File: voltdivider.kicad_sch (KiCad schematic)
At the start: 20 parts, among them J1 Conn_01x01_Pin, J7 Conn_01x01_Pin, J8 Conn_01x01_Pin, SW1 SW_Rotary_1x8_MP

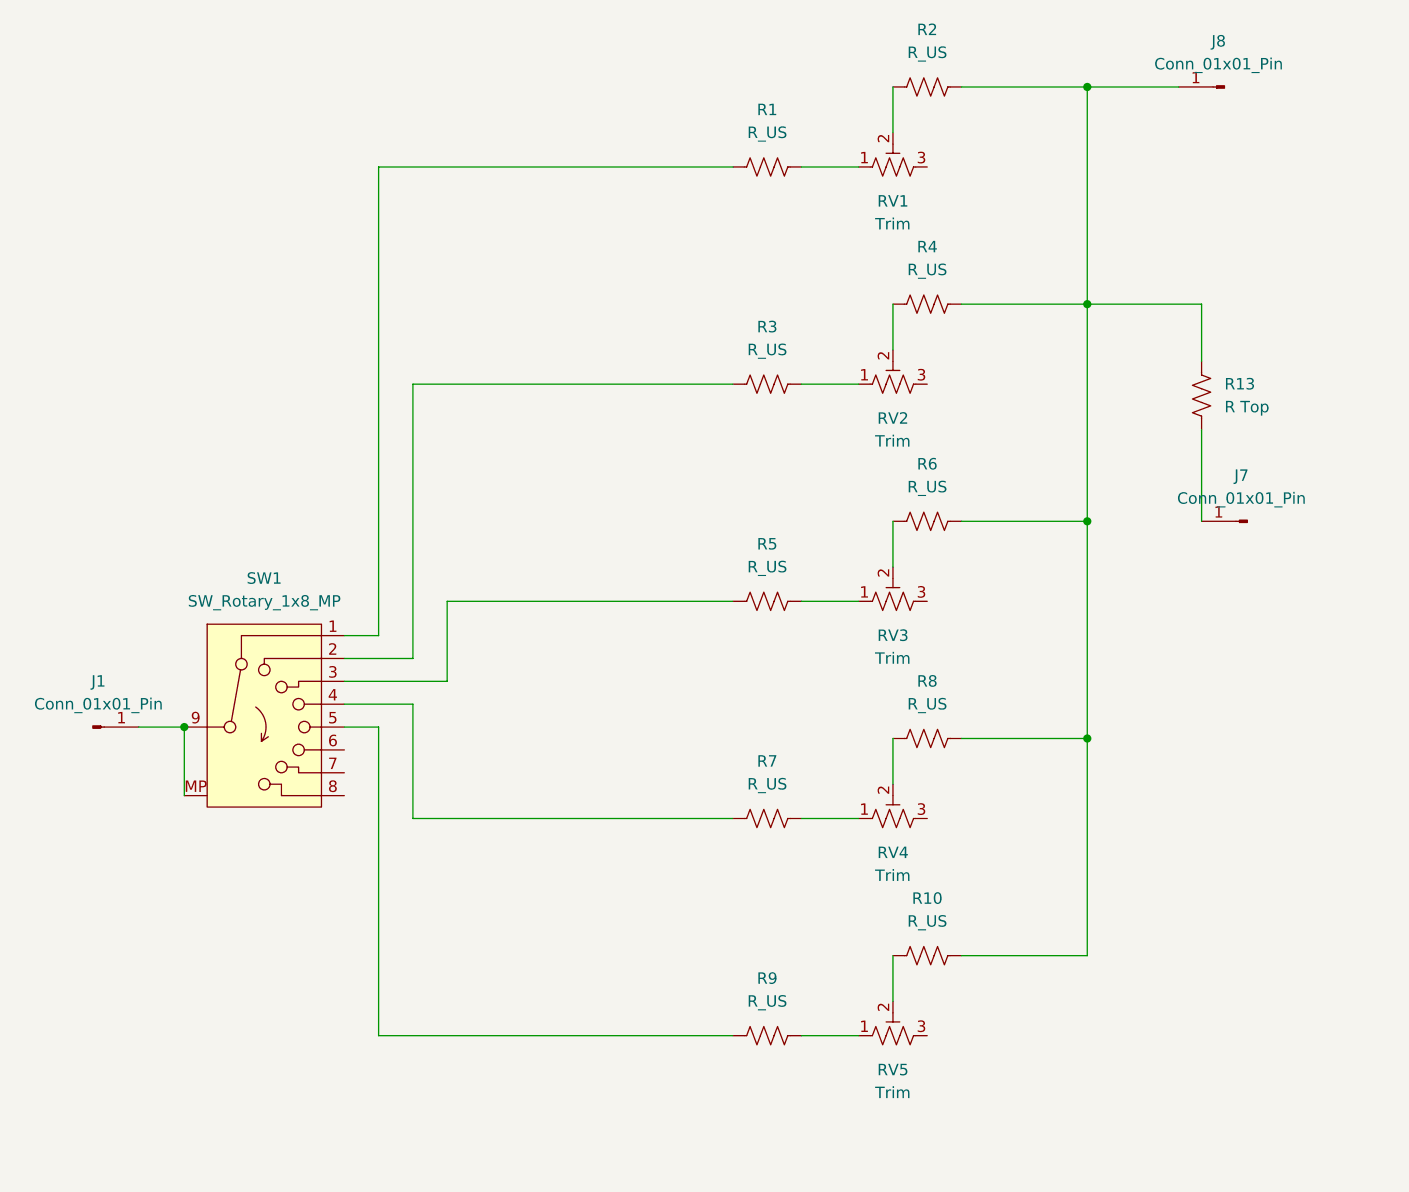
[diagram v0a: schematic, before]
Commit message: creating documentation
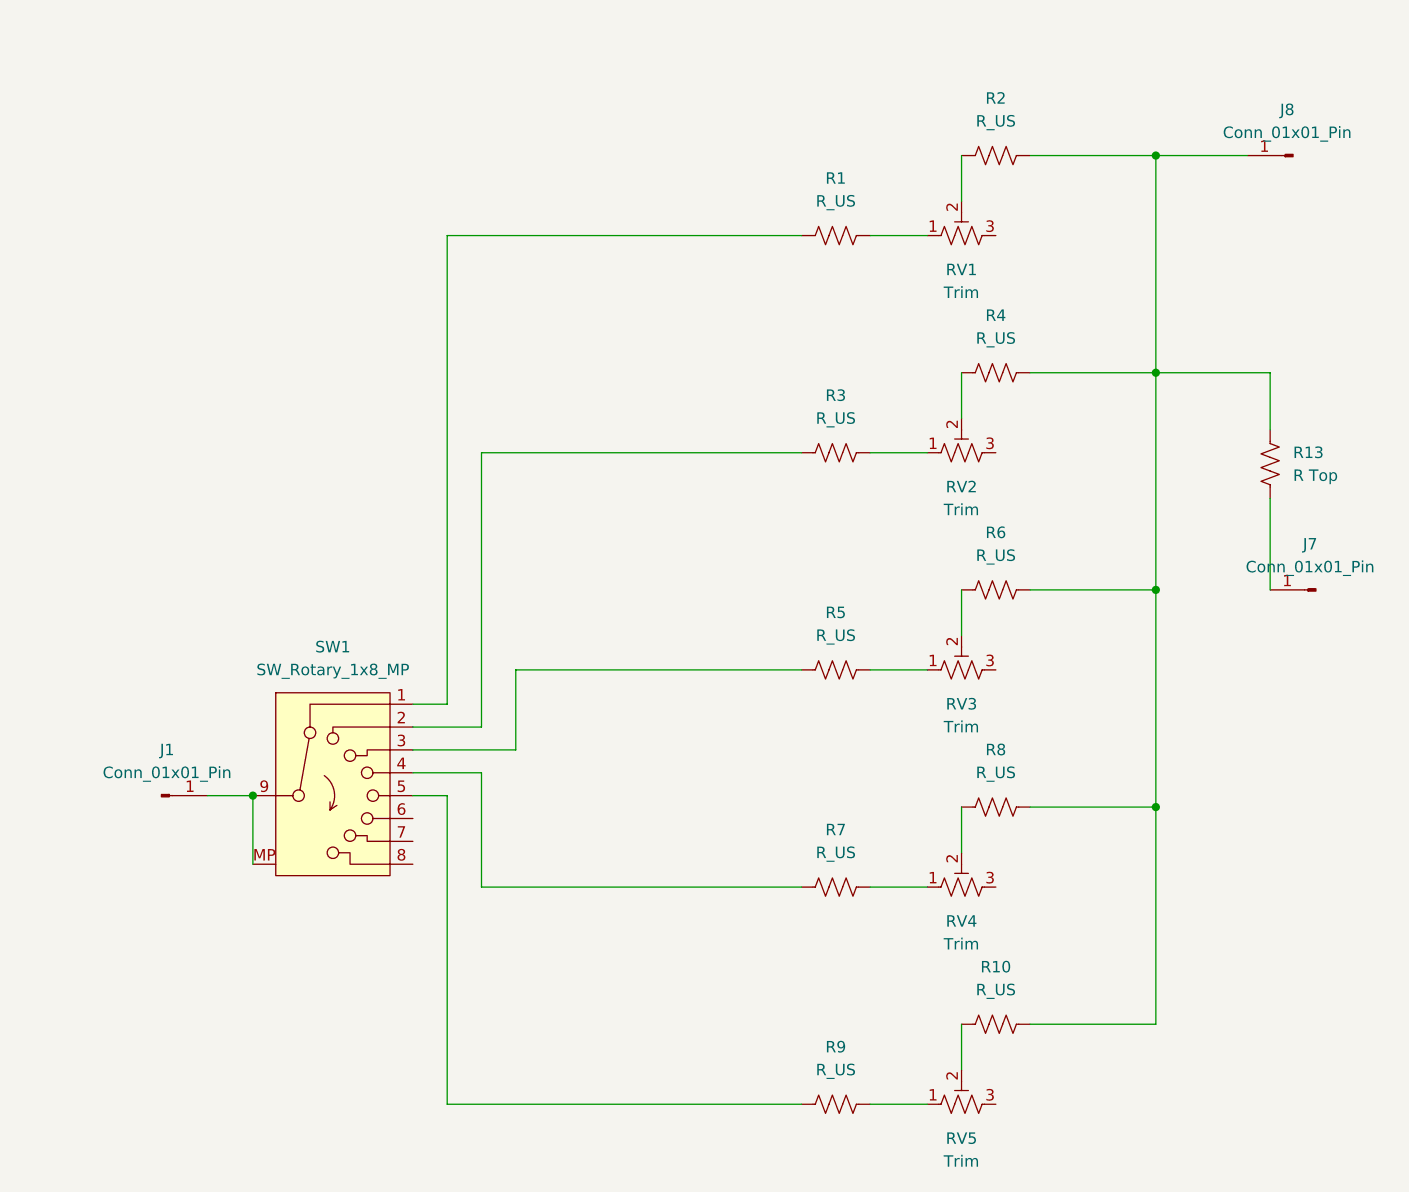
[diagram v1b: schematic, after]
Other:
- company: (none) -> Hucklecat
- title: (none) -> Switchable Voltage Divider
- moved on the sheet: J1, J7, J8, R1, R10, R13, R2, R3, R4, R5, R6, R7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
